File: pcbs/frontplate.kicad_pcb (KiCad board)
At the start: 2 copper layers, 133.3 x 91.7 mm, 5 parts

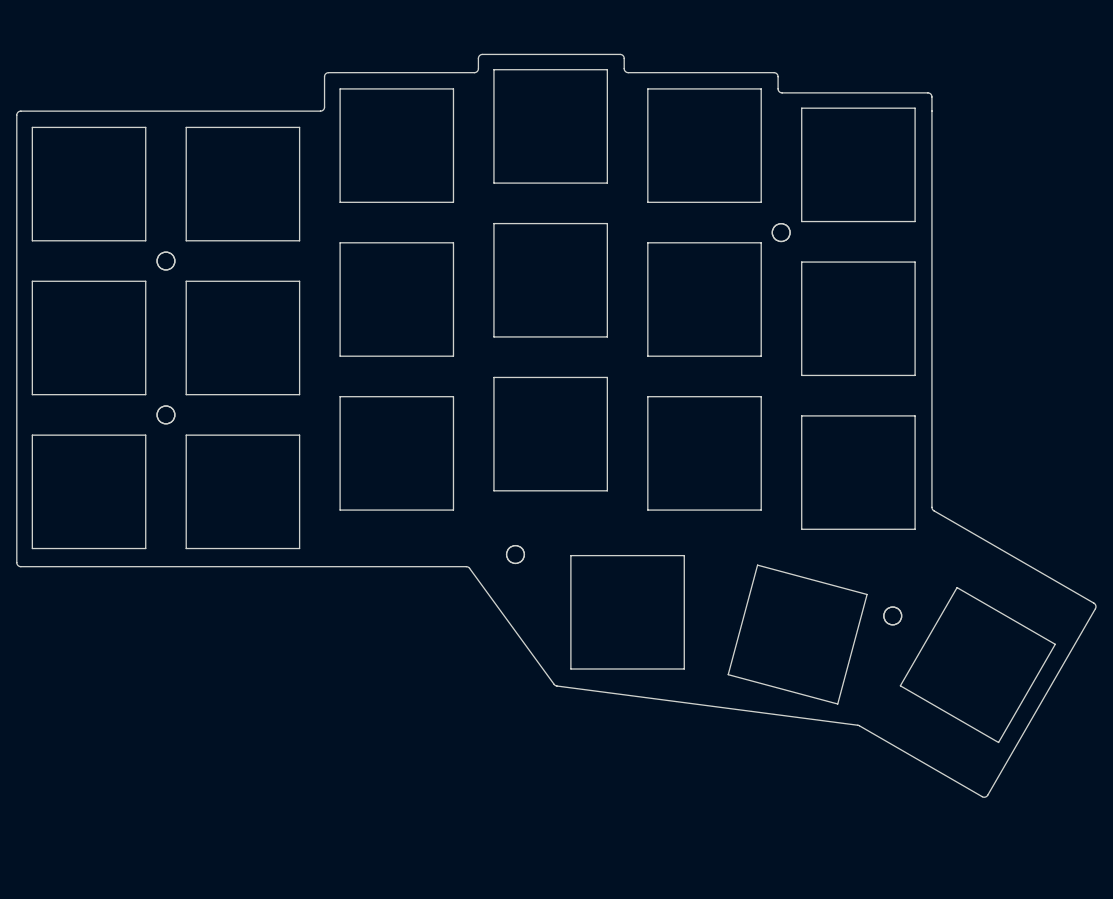
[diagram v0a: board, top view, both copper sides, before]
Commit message: First commit? Second?
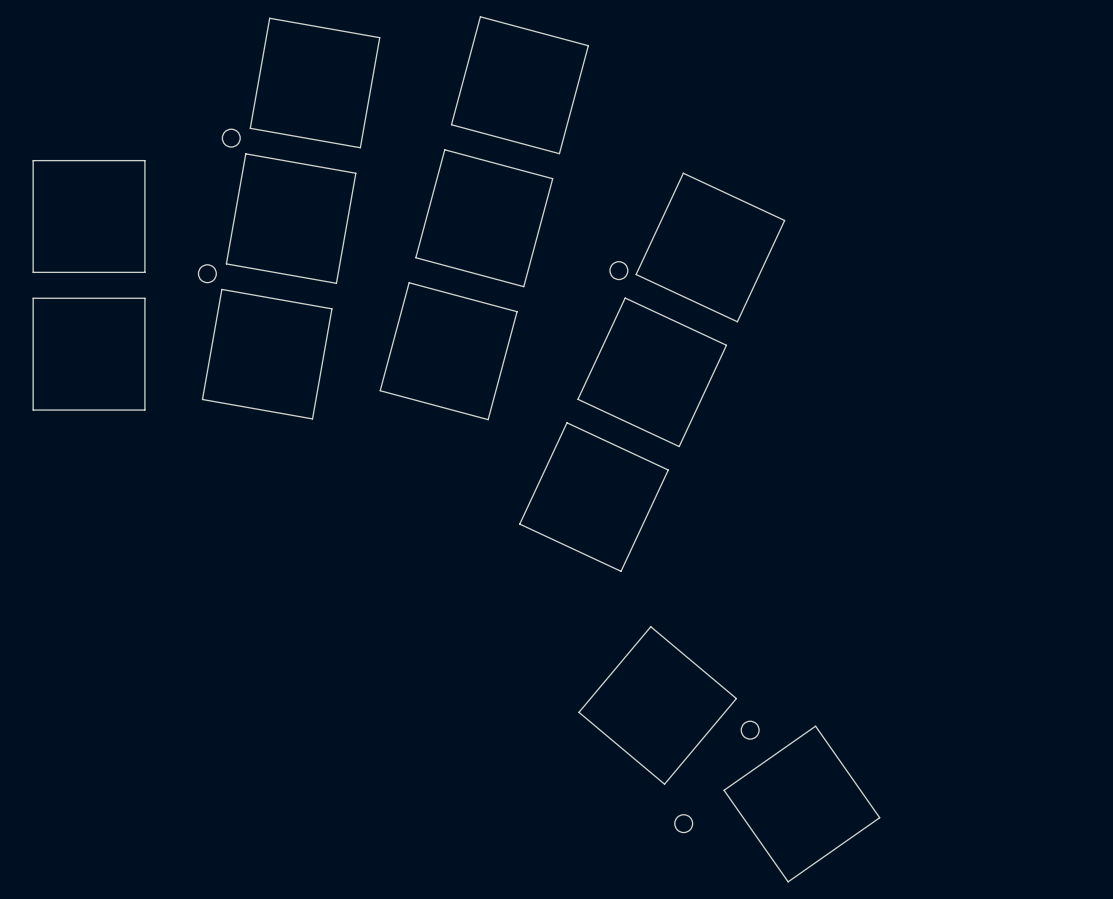
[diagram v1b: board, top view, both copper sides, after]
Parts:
- moved MH4 39.2 mm to (173.4, 141.0), turned to 35 degrees
- moved MH5 22.6 mm to (181.6, 129.4), turned to 35 degrees
- moved MH3 20.6 mm to (165.4, 72.7), turned to -25 degrees
- moved MH2 18.2 mm to (114.6, 73.1), turned to -10 degrees
- moved MH1 17.2 mm to (117.6, 56.3), turned to -10 degrees
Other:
- board size 133.3 x 91.7 mm -> 104.5 x 106.8 mm
